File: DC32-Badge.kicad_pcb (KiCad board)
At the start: 2 copper layers, 37 parts, among them J1 Conn_01x06, J2 Hirose_FH34-SRJ-24S, J3 Conn_01x06, J4 Conn_01x06, J5 Micro_SD_Card_Det, P1 2479, Q1 RTF025N03TL, SW1 SW_Push_DPDT, SW2 SW_Push_DPDT, SW3 SW_Push, SW4 SW_Push, U1 ESP32-C3-MINI-1, U2 AP2112K-3.3

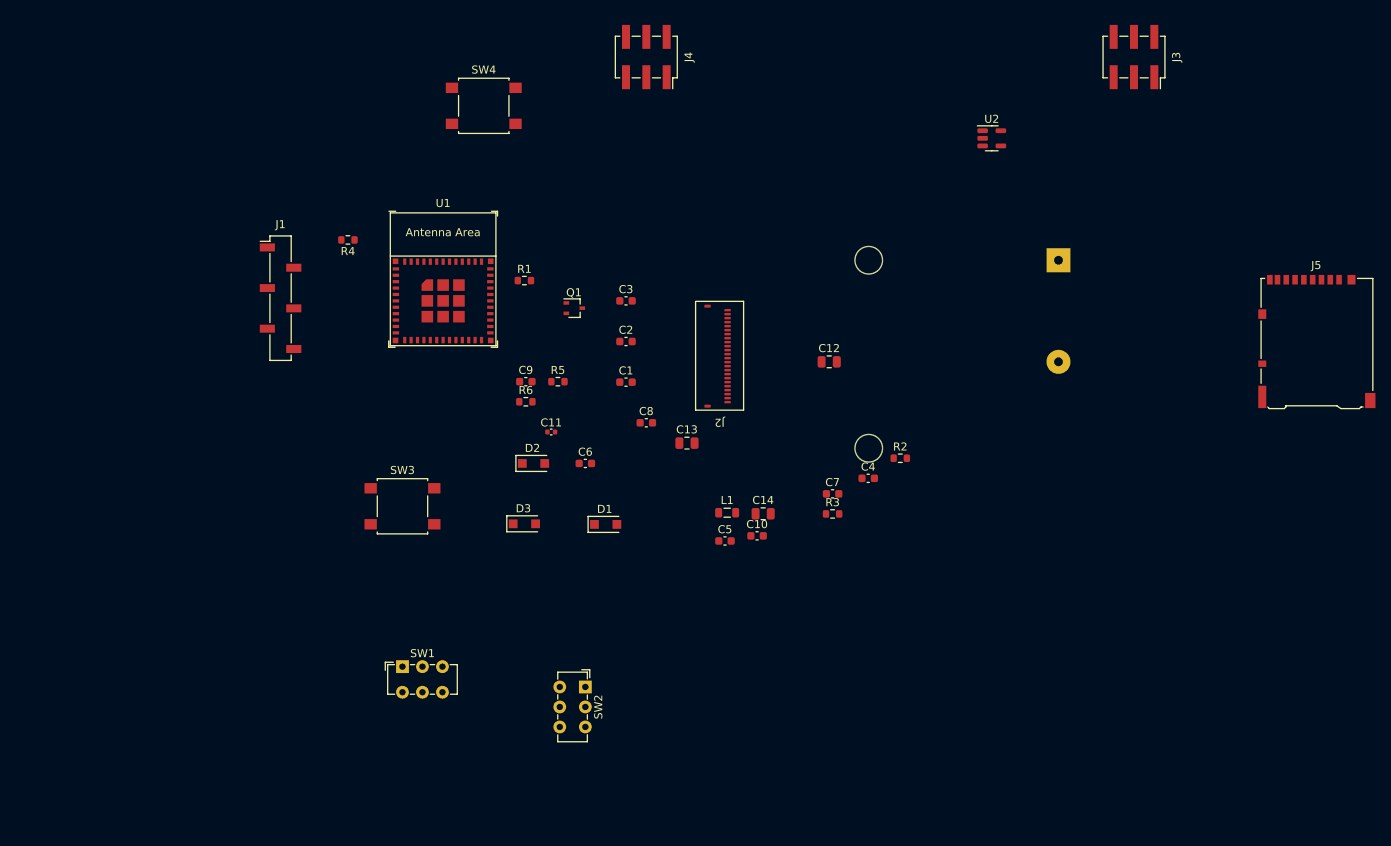
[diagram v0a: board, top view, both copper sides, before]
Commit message: Initial place and route.
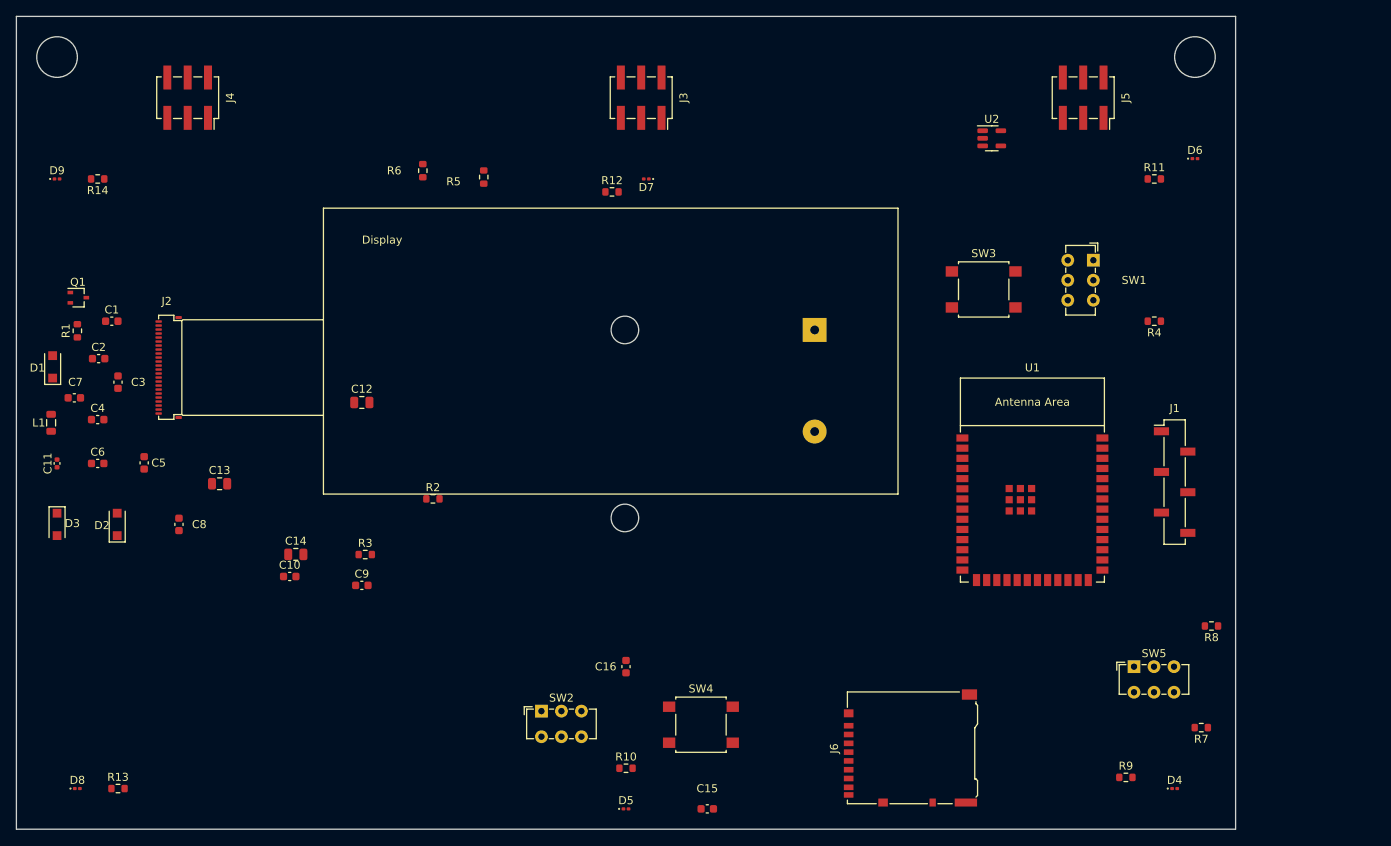
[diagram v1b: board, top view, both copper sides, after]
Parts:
- added C15: 1uF/25V, Capacitor_SMD:C_0603_1608Metric, F.Cu at (116.8, 121.9)
- added C16: 1uF/25V, Capacitor_SMD:C_0603_1608Metric, F.Cu at (106.7, 104.1)
- added D4: LED, LED_SMD:LED_0201_0603Metric, F.Cu at (175.3, 119.4)
- added D5: LED, LED_SMD:LED_0201_0603Metric, F.Cu at (106.7, 121.9)
- added D6: LED, LED_SMD:LED_0201_0603Metric, F.Cu at (177.8, 40.6)
- added D7: LED, LED_SMD:LED_0201_0603Metric, F.Cu at (109.2, 43.2)
- added D8: LED, LED_SMD:LED_0201_0603Metric, F.Cu at (38.1, 119.4)
- added D9: LED, LED_SMD:LED_0201_0603Metric, F.Cu at (35.6, 43.2)
- added J5: Conn_01x06, Connector_PinSocket_2.54mm:PinSocket_2x03_P2.54mm_Vertical_SMD, F.Cu at (163.8, 33.0)
- added R10: 1k, Resistor_SMD:R_0603_1608Metric, F.Cu at (106.7, 116.8)
- added R11: 1k, Resistor_SMD:R_0603_1608Metric, F.Cu at (172.7, 43.2)
- added R12: 1k, Resistor_SMD:R_0603_1608Metric, F.Cu at (104.9, 44.8)
- added R13: 1k, Resistor_SMD:R_0603_1608Metric, F.Cu at (43.2, 119.4)
- added R14: 1k, Resistor_SMD:R_0603_1608Metric, F.Cu at (40.6, 43.2)
- added R7: 10k, Resistor_SMD:R_0603_1608Metric, F.Cu at (178.6, 111.8)
- added R8: 10k, Resistor_SMD:R_0603_1608Metric, F.Cu at (179.9, 99.1)
- added R9: 1k, Resistor_SMD:R_0603_1608Metric, F.Cu at (169.2, 118.0)
- added SW5: PROGRAM, Button_Switch_THT:SW_E-Switch_EG1271_SPDT, F.Cu at (170.2, 104.1)
- J2: footprint HiroseElectricCo:FH34SRJ-24S -> HiroseElectricCo:E2266QS0F1
- SW2: value SW_Push_DPDT -> EVIL_SWITCH
- U1: value ESP32-C3-MINI-1 -> ESP32-S3-WROOM-1; footprint Espressif:ESP32-C3-MINI-1 -> Espressif:ESP32-S3-WROOM-1
- moved J1 114.1 mm to (175.3, 81.1)
- moved R4 101.3 mm to (172.7, 61.0)
- moved SW1 100.2 mm to (165.1, 53.3), turned to -90 degrees
- moved C4 96.6 mm to (40.6, 73.3)
- moved C7 95.5 mm to (37.7, 70.5), turned to 180 degrees
- moved L1 85.2 mm to (34.8, 73.7), turned to 90 degrees
- moved SW4 82.0 mm to (116.0, 111.4)
- moved U1 77.9 mm to (157.5, 83.8)
- moved SW3 77.5 mm to (151.4, 57.0)
- moved C5 73.3 mm to (46.5, 78.7), turned to -90 degrees
- moved D1 71.9 mm to (35.0, 66.7), turned to 90 degrees
- moved J6 71.8 mm to (142.2, 114.3), turned to 90 degrees
- moved J2 71.1 mm to (48.3, 66.0), turned to 0 degrees
- moved C2 66.0 mm to (40.8, 65.6)
- moved C1 64.7 mm to (42.4, 61.0)
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- renumbered J5 to J6
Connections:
- C11 pad 2: Net-(C8-Pad2) -> +3.3V
- C14 pad 2: Net-(C8-Pad2) -> +3.3V
- C8 pad 2: Net-(C8-Pad2) -> +3.3V
- C9 pad 2: Net-(U1-Pad8) -> RST
- J1 pad 2: Net-(J1-Pad2) -> PROG_TX
- J1 pad 3: Net-(J1-Pad3) -> PROG_RX
- J2 pad 12: Net-(U1-Pad26) -> Net-(J2-Pad12)
- J2 pad 14: Net-(U1-Pad21) -> Net-(J2-Pad14)
- J2 pad 15: Net-(C8-Pad2) -> +3.3V
- J2 pad 16: Net-(C8-Pad2) -> +3.3V
- J3 pad 3: Net-(U1-Pad19) -> SDA
- J3 pad 4: Net-(U1-Pad18) -> SCL
- J3 pad 6: Net-(C8-Pad2) -> +3.3V
- J4 pad 3: Net-(U1-Pad19) -> SDA
- J4 pad 4: Net-(U1-Pad18) -> SCL
- J4 pad 6: Net-(C8-Pad2) -> +3.3V
- J6 pad 2: Net-(U1-Pad6) -> Net-(U1-Pad12)
- J6 pad 3: Net-(U1-Pad21) -> Net-(J2-Pad14)
- J6 pad 4: Net-(C8-Pad2) -> +3.3V
- J6 pad 7: Net-(U1-Pad5) -> Net-(J6-Pad7)
- L1 pad 1: Net-(C8-Pad2) -> +3.3V
- R2 pad 1: Net-(C8-Pad2) -> +3.3V
- R2 pad 2: Net-(U1-Pad27) -> EVIL
- R3 pad 1: Net-(U1-Pad8) -> +3.3V
- R3 pad 2: Net-(C8-Pad2) -> RST
- R4 pad 1: Net-(U1-Pad23) -> +3.3V
- R4 pad 2: Net-(C8-Pad2) -> SW_PUSH
- R5 pad 1: Net-(C8-Pad2) -> +3.3V
- R5 pad 2: Net-(U1-Pad18) -> SCL
- R6 pad 1: Net-(C8-Pad2) -> +3.3V
- R6 pad 2: Net-(U1-Pad19) -> SDA
- SW2 pad 2: Net-(U1-Pad27) -> EVIL
- SW3 pad 1: Net-(U1-Pad8) -> RST
- SW4 pad 2: Net-(U1-Pad23) -> SW_PUSH
- U1 pad 10: unconnected-(U1-Pad10) -> LED6
- U1 pad 11: GND -> Net-(J2-Pad12)
- U1 pad 12: Net-(J2-Pad10) -> Net-(U1-Pad12)
- U1 pad 13: Net-(J2-Pad9) -> EVIL
- U1 pad 14: GND -> unconnected-(U1-Pad14)
- U1 pad 15: unconnected-(U1-Pad15) -> LED2
- U1 pad 16: Net-(J2-Pad8) -> PROG_GPIO46
- U1 pad 17: unconnected-(U1-Pad17) -> SW_PUSH
- U1 pad 18: Net-(U1-Pad18) -> Net-(J2-Pad8)
- U1 pad 19: Net-(U1-Pad19) -> Net-(J2-Pad9)
- U1 pad 2: GND -> +3.3V
- U1 pad 20: Net-(J2-Pad13) -> Net-(J2-Pad10)
- U1 pad 21: Net-(U1-Pad21) -> Net-(J2-Pad11)
- U1 pad 22: Net-(J2-Pad11) -> LED3
- U1 pad 23: Net-(U1-Pad23) -> unconnected-(U1-Pad23)
- U1 pad 26: Net-(U1-Pad26) -> unconnected-(U1-Pad26)
- U1 pad 27: Net-(U1-Pad27) -> PROG_GPIO0
- U1 pad 3: Net-(C8-Pad2) -> RST
- U1 pad 30: Net-(J1-Pad3) -> unconnected-(U1-Pad30)
- U1 pad 31: Net-(J1-Pad2) -> unconnected-(U1-Pad31)
- U1 pad 36: GND -> PROG_RX
- U1 pad 4: unconnected-(U1-Pad4) -> SCL
- U1 pad 5: Net-(U1-Pad5) -> SDA
- U1 pad 6: Net-(U1-Pad6) -> Net-(J2-Pad13)
- U1 pad 7: unconnected-(U1-Pad7) -> Net-(J2-Pad14)
- U1 pad 8: Net-(U1-Pad8) -> LED4
- U1 pad 9: unconnected-(U1-Pad9) -> LED5
- U2 pad 5: Net-(C8-Pad2) -> +3.3V
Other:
- board outline added: 152.4 x 101.6 mm
